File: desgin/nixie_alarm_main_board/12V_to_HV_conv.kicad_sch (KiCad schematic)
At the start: 19 parts, among them IC1 LM3488MM, IC5 TPH5200FNH, IC8 MCP4018T-502E_LT

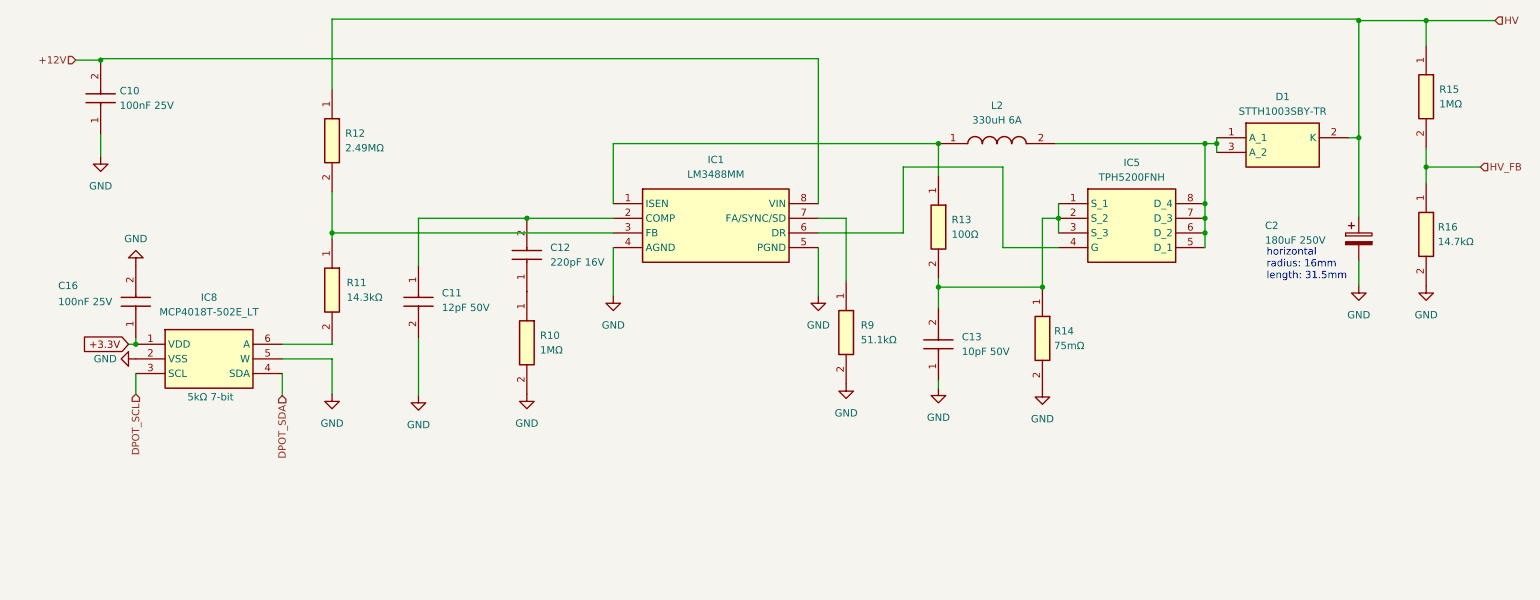
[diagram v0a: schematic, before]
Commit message: filter caps
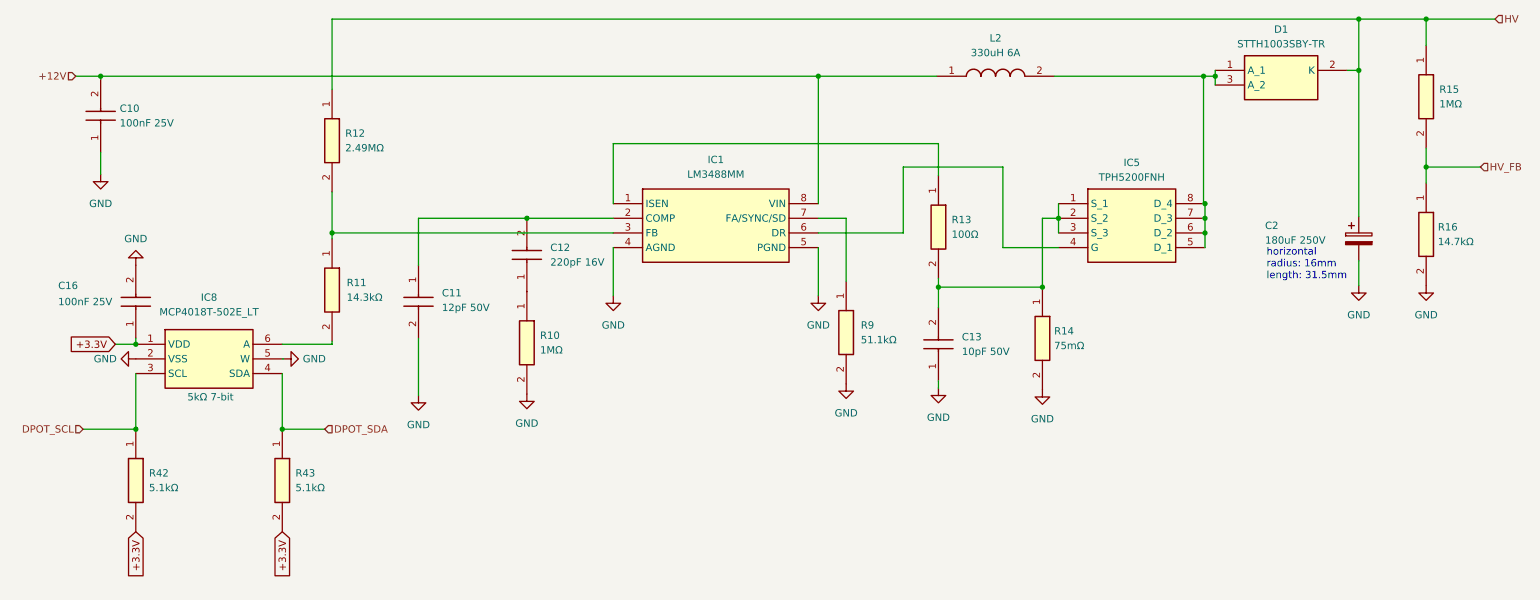
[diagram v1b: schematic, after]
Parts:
- added R42, R43: 5.1kΩ, RESC2012X60N, symbol SamacSys_Parts:ERJ-UP6D5101V
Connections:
- net +12V: now also L2.1
- net +3.3V: now also R42.2, R43.2
- net DPOT_SCL: now also R42.1
- net DPOT_SDA: now also R43.1
- net at IC1.1 (ISEN), R13.1: no longer L2.1
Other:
- moved on the sheet: C10, D1, L2
